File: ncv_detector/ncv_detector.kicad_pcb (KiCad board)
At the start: 2 copper layers, 106.5 x 38 mm, 10 parts, among them Q1 2N3904, Q2 2N3904, Q3 2N3904

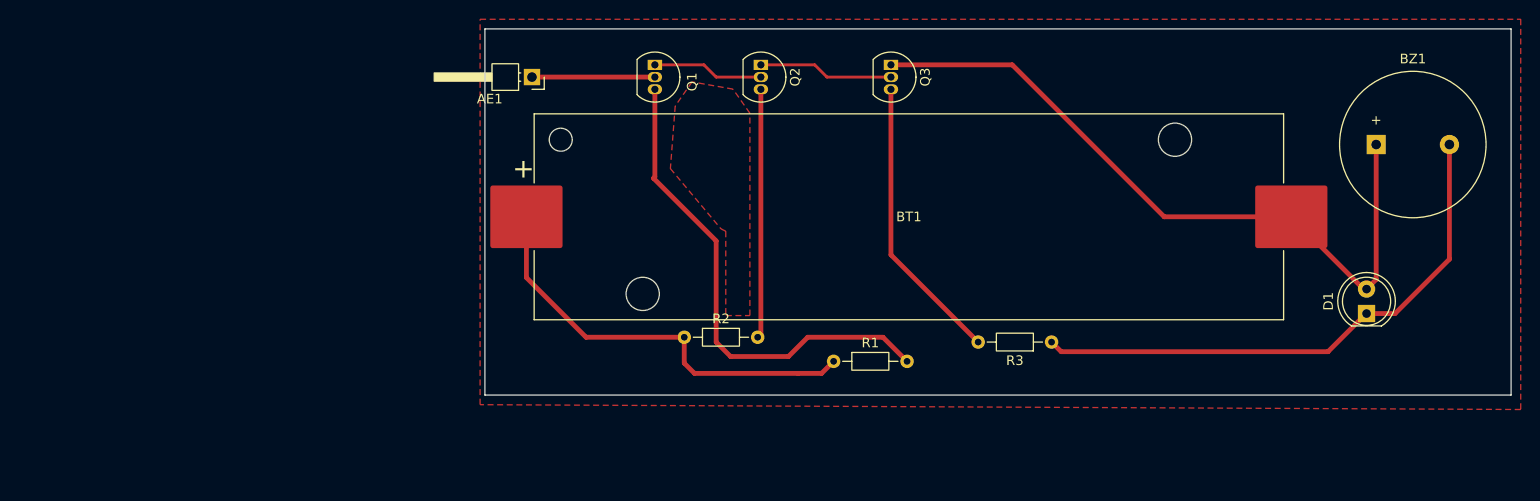
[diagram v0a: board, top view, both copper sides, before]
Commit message: screenshot added
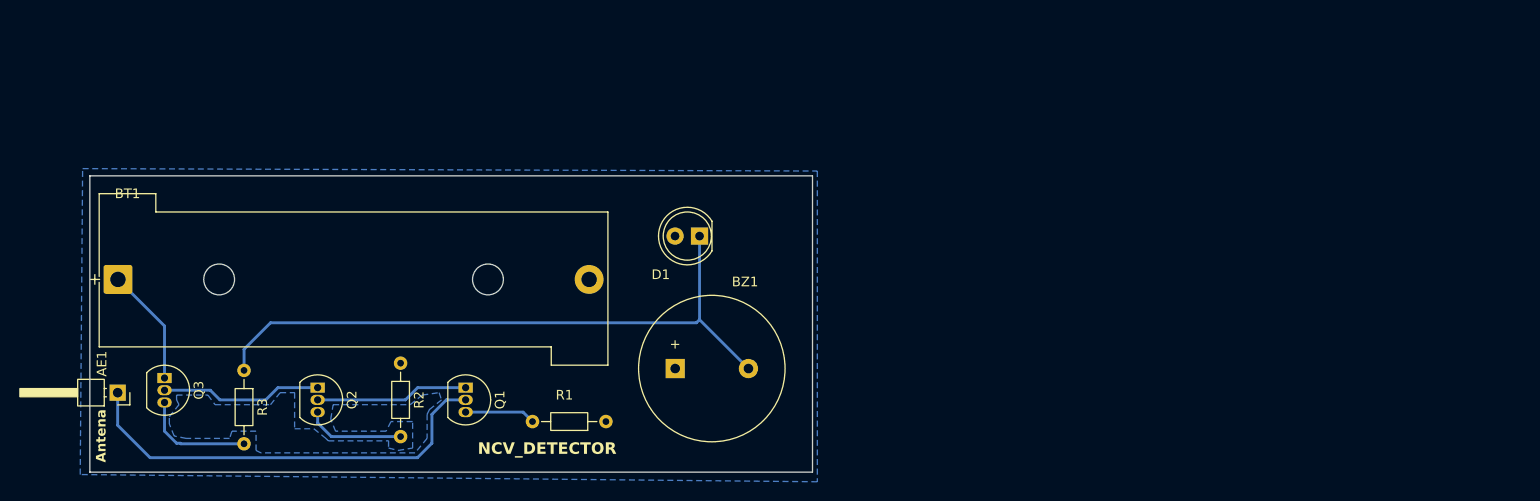
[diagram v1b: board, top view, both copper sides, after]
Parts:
- added REF**: KiCad-Logo2_12mm_SilkScreen, Symbol:KiCad-Logo2_12mm_SilkScreen, B.Cu at (107.8, 102.3)
- BT1: footprint Battery:BatteryHolder_Keystone_1042_1x18650 -> Battery:BatteryHolder_Bulgin_BX0034_1xAAA
- moved R3 83.9 mm to (93.0, 111.9), turned to -90 degrees
- moved BT1 82.3 mm to (79.9, 102.5)
- moved Q3 82.1 mm to (84.8, 112.7)
- moved BZ1 76.4 mm to (137.8, 111.8)
- moved D1 69.7 mm to (140.3, 98.0), turned to 180 degrees
- moved Q2 56.9 mm to (100.6, 113.7)
- moved AE1 54.1 mm to (79.9, 114.2)
- moved Q1 38.8 mm to (116.0, 113.7)
- moved R2 29.6 mm to (109.2, 111.2), turned to -90 degrees
- moved R1 24.4 mm to (130.6, 117.2), turned to 180 degrees
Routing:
- net (no net): track 48.1 -> 0.00 mm
- net Net-(Q1-C): track 51.3 -> 7.35 mm
- net Net-(AE1-A): track 12.8 -> 45.1 mm
- net Net-(BT1-+): track 44.4 -> 12.2 mm
- net GND: track 25.6 -> 0.00 mm
- net Net-(Q3-C): track 30.0 -> 11.8 mm
- net Net-(Q2-C): track 25.9 -> 10.3 mm
- net Net-(BZ1--): track 57.6 -> 66.6 mm
- net Net-(Q1-E): track 11.5 -> 15.9 mm
- net Net-(Q2-E): track 14.0 -> 16.8 mm
- added copper zone on B.Cu, net GND
- removed copper zone on F.Cu, net GND
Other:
- board size 106.5 x 38 mm -> 75 x 30.8 mm
- board text added: "Antena"
- board text added: "NCV_DETECTOR"
